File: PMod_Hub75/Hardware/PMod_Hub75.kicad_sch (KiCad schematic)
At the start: 13 parts, among them IC1 SN74LVC8T245DWR, IC2 SN74LVC8T245DWR, J1 Conn_02x06_Counter_Clockwise, J2 Conn_02x06_Counter_Clockwise, J3 Conn_02x08_Counter_Clockwise

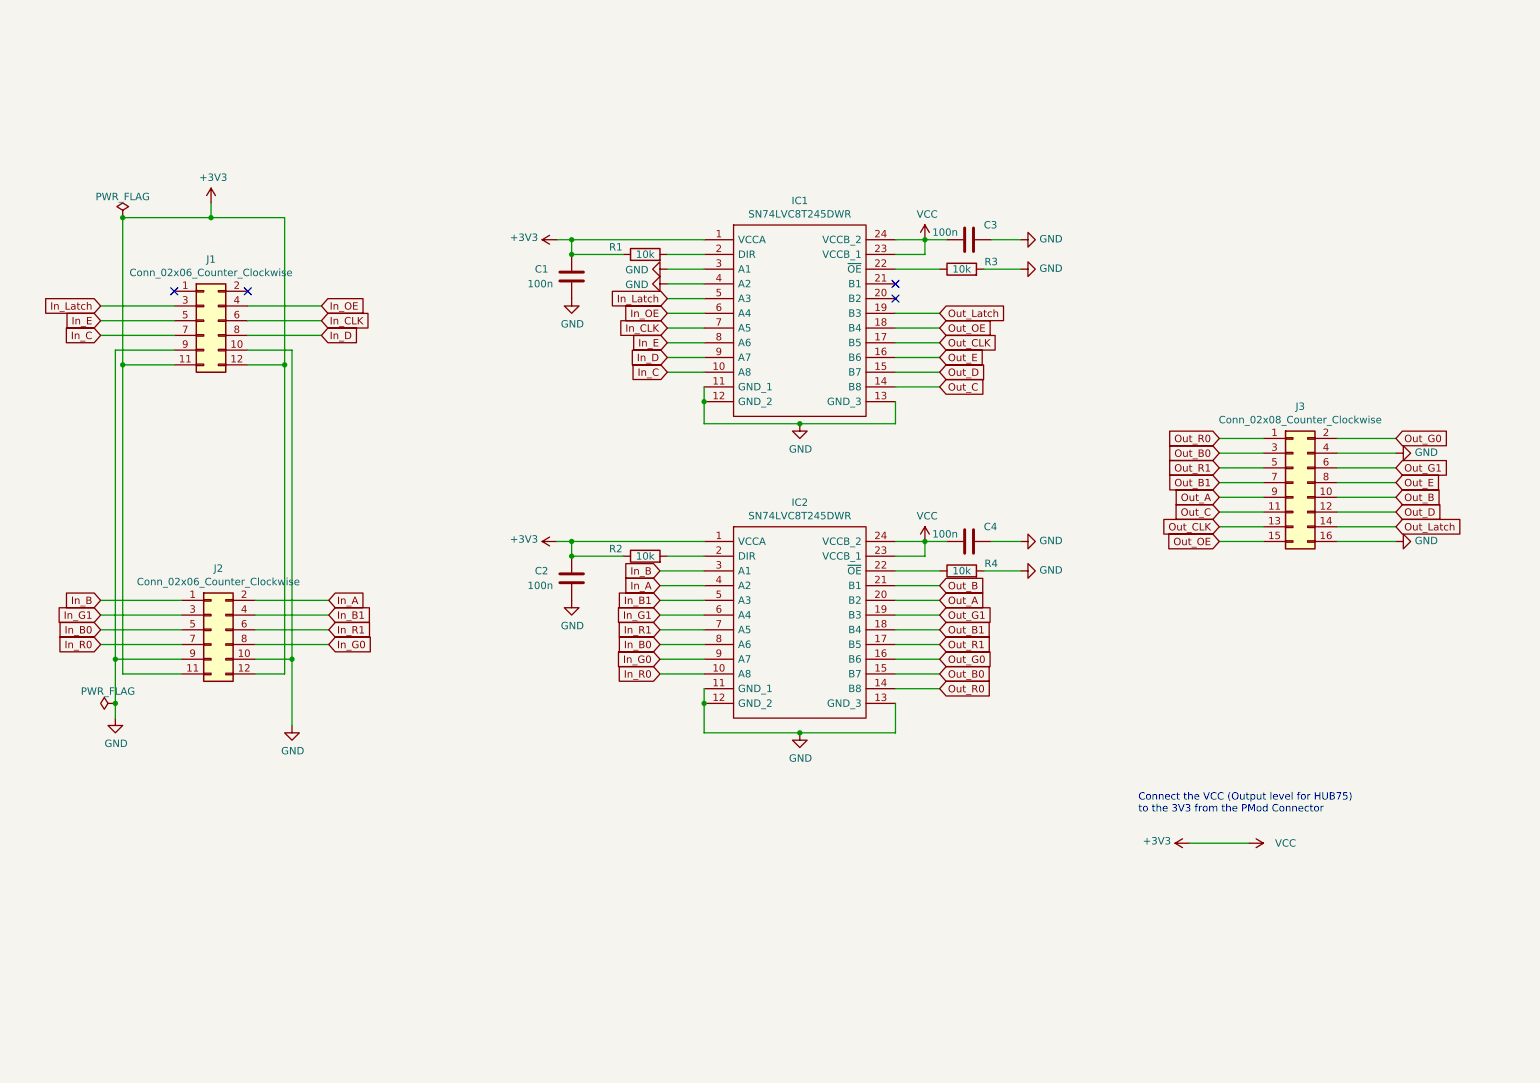
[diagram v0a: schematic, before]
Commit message: Tidy up the schematic and add titles
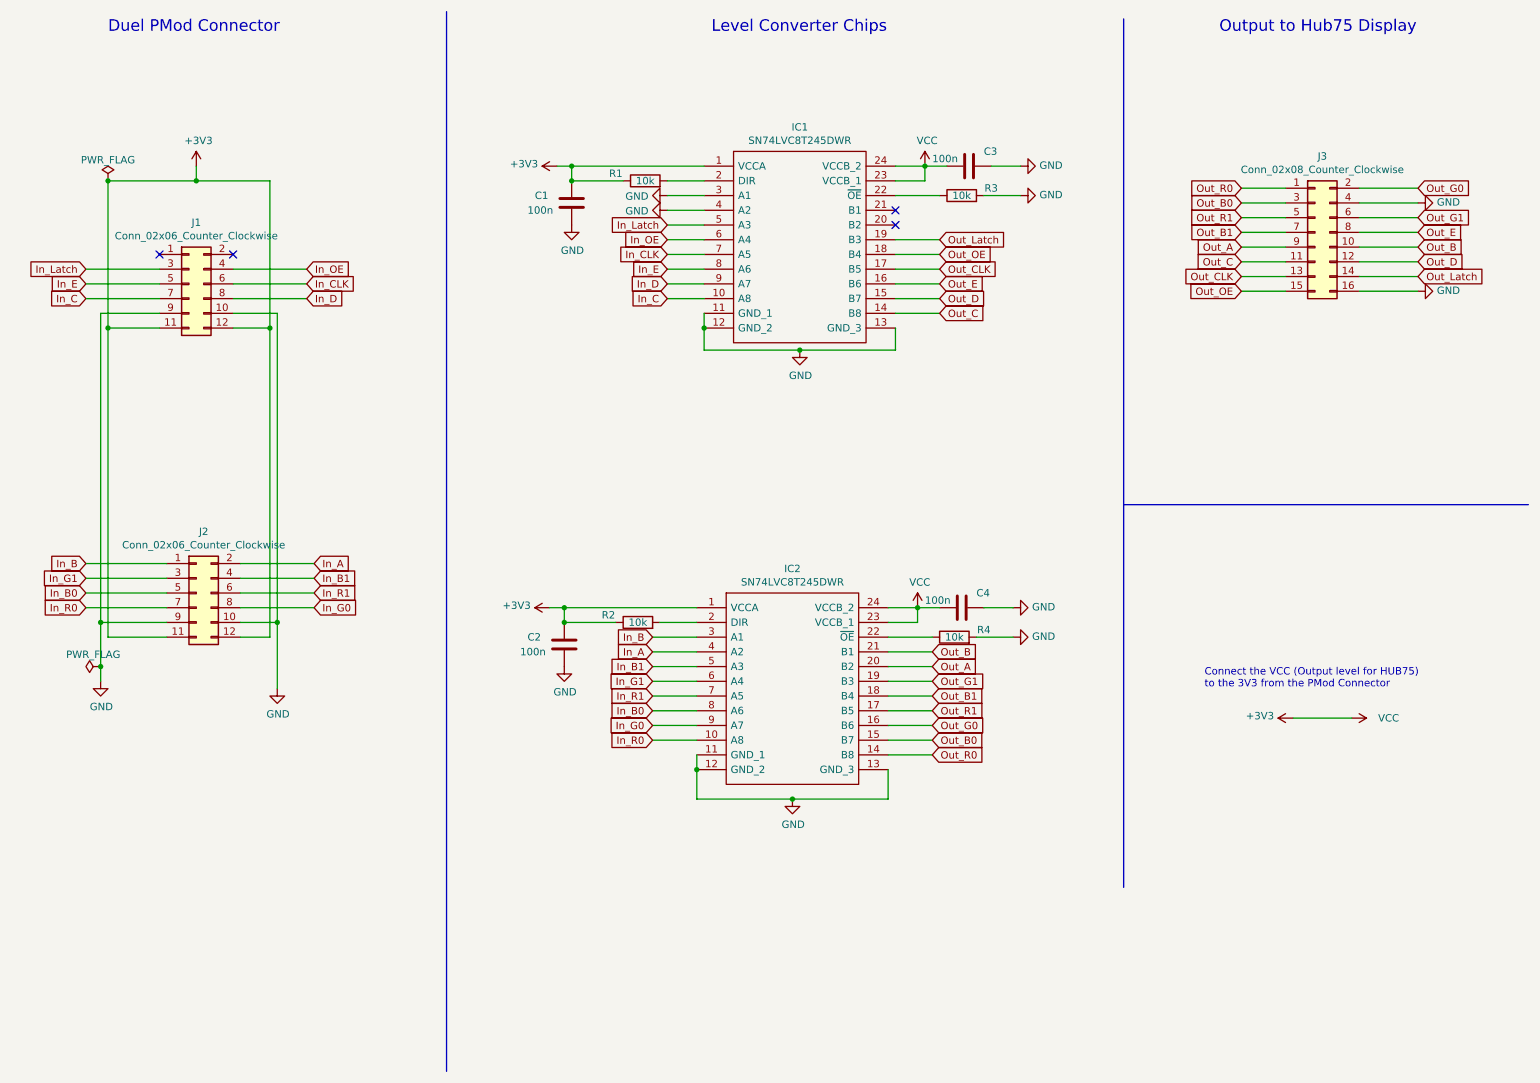
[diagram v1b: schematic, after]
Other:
- note added: "Duel PMod Connector"
- note added: "Level Converter Chips"
- note added: "Output to Hub75 Display"
- moved on the sheet: C1, C2, C3, C4, IC1, IC2, J1, J2, J3, R1, R2, R3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

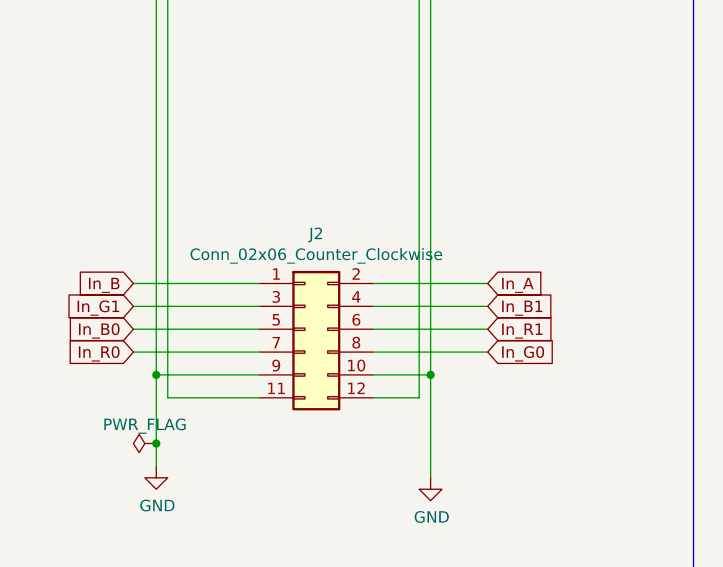
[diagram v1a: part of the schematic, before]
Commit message: Swap A and B pins so they are in order for the RP2040 code
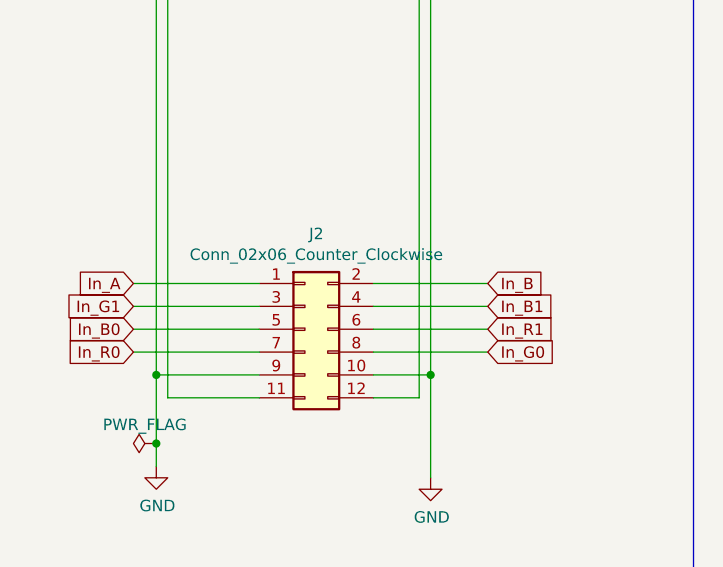
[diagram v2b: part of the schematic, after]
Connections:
- net In_A: now also J2.1 (Pin_1); no longer J2.2 (Pin_2)
- net In_B: now also J2.2 (Pin_2); no longer J2.1 (Pin_1)
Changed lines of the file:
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@@
     )
   )
-  (global_label "In_B" (shape input) (at 35.56 107.95 180) (fields_autoplaced)
-    (effects (font (size 1.27 1.27)) (justify right))
-    (property "Intersheet References" "${INTERSHEET_REFS}" (id 0) (at -2.54 -6.35 0)
+  (global_label "In_B" (shape input) (at 74.93 107.95 0) (fields_autoplaced)
+    (effects (font (size 1.27 1.27)) (justify left))
+    (property "Intersheet References" "${INTERSHEET_REFS}" (id 0) (at 113.03 222.25 0)
       (effects (font (size 1.27 1.27)) hide)
     )
@@
     )
   )
-  (global_label "In_A" (shape input) (at 74.93 107.95 0) (fields_autoplaced)
-    (effects (font (size 1.27 1.27)) (justify left))
-    (property "Intersheet References" "${INTERSHEET_REFS}" (id 0) (at -2.54 -6.35 0)
+  (global_label "In_A" (shape input) (at 35.56 107.95 180) (fields_autoplaced)
+    (effects (font (size 1.27 1.27)) (justify right))
+    (property "Intersheet References" "${INTERSHEET_REFS}" (id 0) (at 113.03 222.25 0)
       (effects (font (size 1.27 1.27)) hide)
     )
@@
   (symbol (lib_id "power:PWR_FLAG") (at 38.1 125.73 90) (unit 1)
     (in_bom yes) (on_board yes) (fields_autoplaced)
-    (property "Reference" "#FLG?" (id 0) (at 36.195 125.73 0)
+    (property "Reference" "#FLG0102" (id 0) (at 36.195 125.73 0)
       (effects (font (size 1.27 1.27)) hide)
     )
@@
     )
     (path "/9545bfbf-48dd-4146-8d60-6fa543402f0a"
-      (reference "#FLG?") (unit 1) (value "PWR_FLAG") (footprint "")
+      (reference "#FLG0102") (unit 1) (value "PWR_FLAG") (footprint "")
     )
     (path "/00000000-0000-0000-0000-000061c461d7"
